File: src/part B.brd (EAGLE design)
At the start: 41 x 75.5 mm, 0 parts

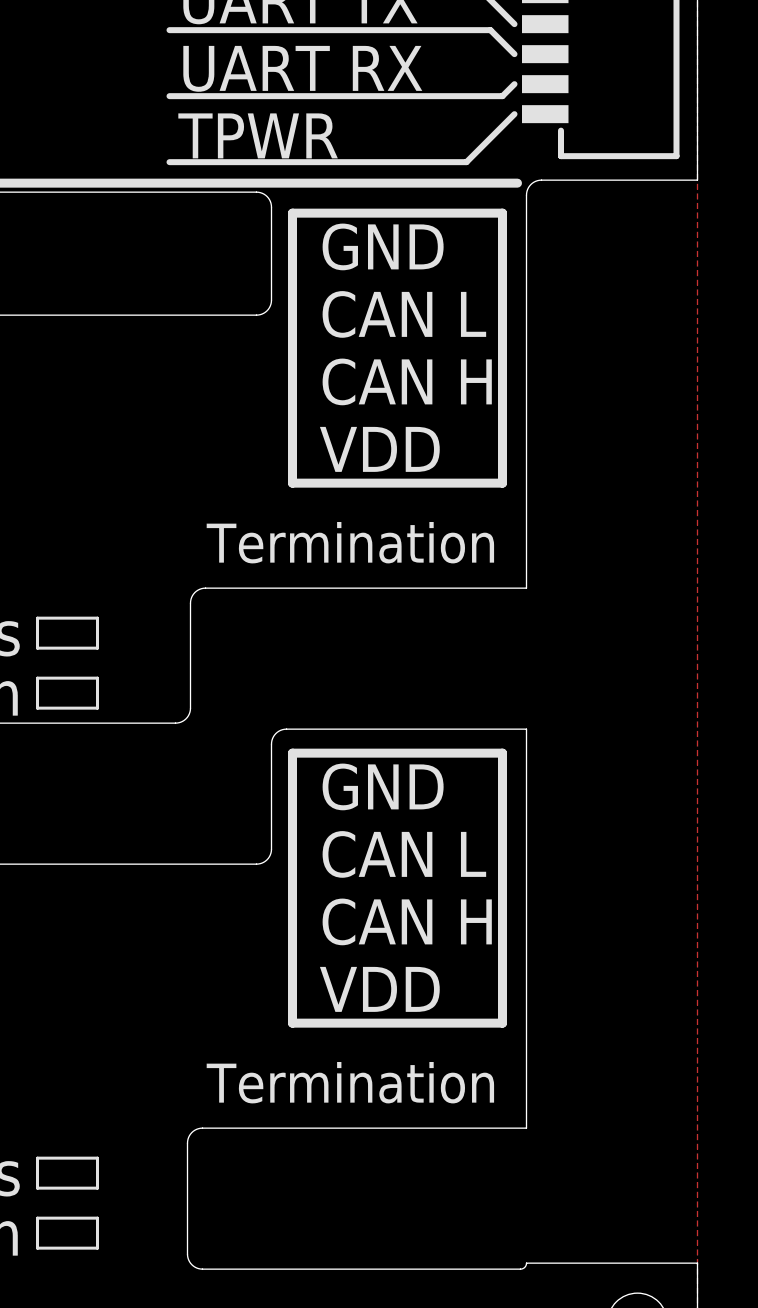
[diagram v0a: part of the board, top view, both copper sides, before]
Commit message: Minor tweaks
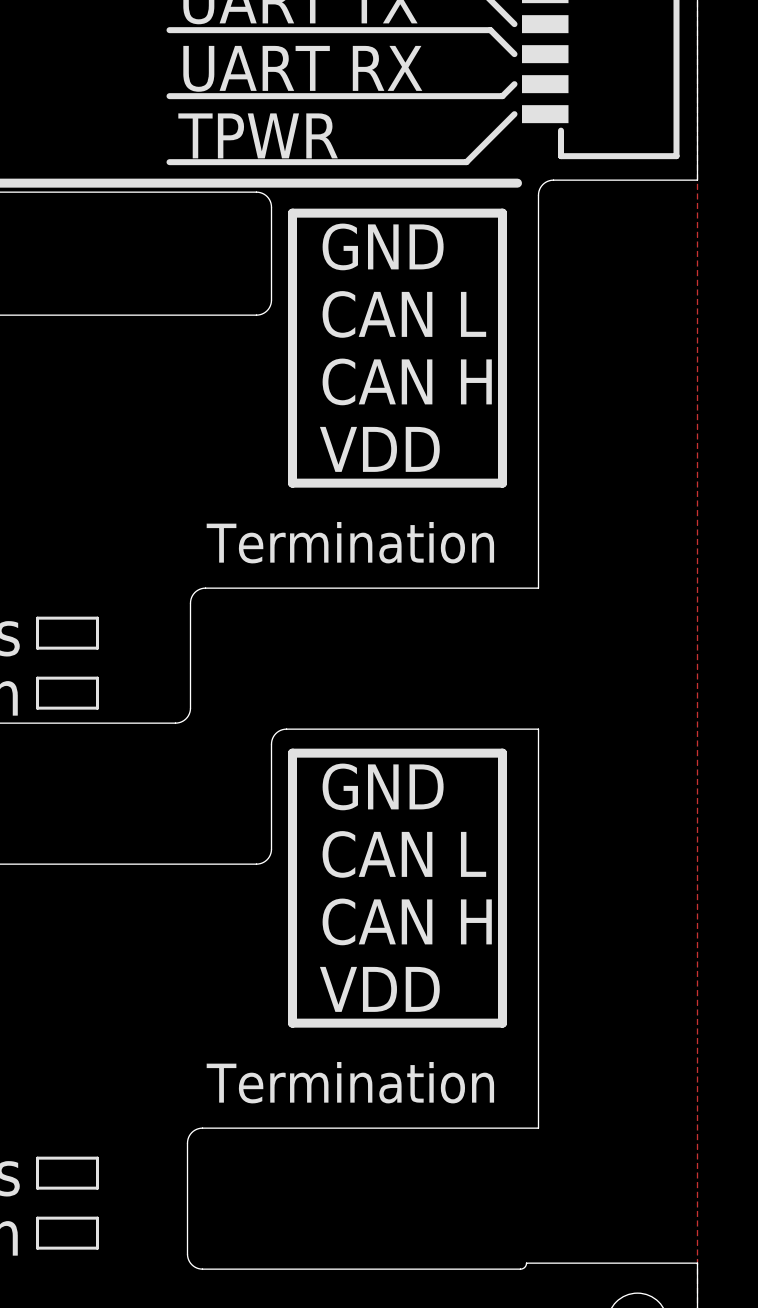
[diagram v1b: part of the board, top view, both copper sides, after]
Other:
- outline, holes or cut-outs redrawn
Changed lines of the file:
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@@
 <setting verticaltext="up"/>
 </settings>
-<grid distance="1" unitdist="mm" unit="mm" style="lines" multiple="1" display="yes" altdistance="5" altunitdist="mil" altunit="mil"/>
+<grid distance="0.4" unitdist="mm" unit="mm" style="lines" multiple="1" display="yes" altdistance="5" altunitdist="mil" altunit="mil"/>
 <layers>
-<layer number="1" name="Top" color="4" fill="1" visible="yes" active="yes"/>
+<layer number="1" name="Top" color="4" fill="1" visible="no" active="yes"/>
 <layer number="2" name="Route2" color="16" fill="1" visible="no" active="no"/>
 <layer number="3" name="Route3" color="17" fill="1" visible="no" active="no"/>
@@
 <layer number="14" name="Route14" color="22" fill="1" visible="no" active="no"/>
 <layer number="15" name="Route15" color="23" fill="1" visible="no" active="no"/>
-<layer number="16" name="Bottom" color="1" fill="1" visible="yes" active="yes"/>
-<layer number="17" name="Pads" color="2" fill="1" visible="yes" active="yes"/>
-<layer number="18" name="Vias" color="2" fill="1" visible="yes" active="yes"/>
+<layer number="16" name="Bottom" color="1" fill="1" visible="no" active="yes"/>
+<layer number="17" name="Pads" color="2" fill="1" visible="no" active="yes"/>
+<layer number="18" name="Vias" color="2" fill="1" visible="no" active="yes"/>
 <layer number="19" name="Unrouted" color="6" fill="1" visible="no" active="yes"/>
-<layer number="20" name="Dimension" color="24" fill="1" visible="no" active="yes"/>
-<layer number="21" name="tPlace" color="7" fill="1" visible="yes" active="yes"/>
-<layer number="22" name="bPlace" color="7" fill="1" visible="yes" active="yes"/>
-<layer number="23" name="tOrigins" color="15" fill="1" visible="yes" active="yes"/>
-<layer number="24" name="bOrigins" color="15" fill="1" visible="yes" active="yes"/>
-<layer number="25" name="tNames" color="7" fill="1" visible="yes" active="yes"/>
-<layer number="26" name="bNames" color="7" fill="1" visible="yes" active="yes"/>
-<layer number="27" name="tValues" color="7" fill="1" visible="yes" active="yes"/>
-<layer number="28" name="bValues" color="7" fill="1" visible="yes" active="yes"/>
-<layer number="29" name="tStop" color="7" fill="3" visible="yes" active="yes"/>
-<layer number="30" name="bStop" color="7" fill="6" visible="yes" active="yes"/>
+<layer number="20" name="Dimension" color="24" fill="1" visible="yes" active="yes"/>
+<layer number="21" name="tPlace" color="7" fill="1" visible="no" active="yes"/>
+<layer number="22" name="bPlace" color="7" fill="1" visible="no" active="yes"/>
+<layer number="23" name="tOrigins" color="15" fill="1" visible="no" active="yes"/>
+<layer number="24" name="bOrigins" color="15" fill="1" visible="no" active="yes"/>
+<layer number="25" name="tNames" color="7" fill="1" visible="no" active="yes"/>
+<layer number="26" name="bNames" color="7" fill="1" visible="no" active="yes"/>
+<layer number="27" name="tValues" color="7" fill="1" visible="no" active="yes"/>
+<layer number="28" name="bValues" color="7" fill="1" visible="no" active="yes"/>
+<layer number="29" name="tStop" color="7" fill="3" visible="no" active="yes"/>
+<layer number="30" name="bStop" color="7" fill="6" visible="no" active="yes"/>
 <layer number="31" name="tCream" color="7" fill="4" visible="no" active="yes"/>
 <layer number="32" name="bCream" color="7" fill="5" visible="no" active="yes"/>
@@
 <layer number="37" name="tTest" color="7" fill="1" visible="no" active="yes"/>
 <layer number="38" name="bTest" color="7" fill="1" visible="no" active="yes"/>
-<layer number="39" name="tKeepout" color="4" fill="11" visible="yes" active="yes"/>
-<layer number="40" name="bKeepout" color="1" fill="11" visible="yes" active="yes"/>
-<layer number="41" name="tRestrict" color="4" fill="10" visible="yes" active="yes"/>
-<layer number="42" name="bRestrict" color="1" fill="10" visible="yes" active="yes"/>
-<layer number="43" name="vRestrict" color="2" fill="10" visible="yes" active="yes"/>
+<layer number="39" name="tKeepout" color="4" fill="11" visible="no" active="yes"/>
+<layer number="40" name="bKeepout" color="1" fill="11" visible="no" active="yes"/>
+<layer number="41" name="tRestrict" color="4" fill="10" visible="no" active="yes"/>
+<layer number="42" name="bRestrict" color="1" fill="10" visible="no" active="yes"/>
+<layer number="43" name="vRestrict" color="2" fill="10" visible="no" active="yes"/>
 <layer number="44" name="Drills" color="7" fill="1" visible="no" active="yes"/>
-<layer number="45" name="Holes" color="7" fill="1" visible="yes" active="yes"/>
+<layer number="45" name="Holes" color="7" fill="1" visible="no" active="yes"/>
 <layer number="46" name="Milling" color="3" fill="1" visible="no" active="yes"/>
 <layer number="47" name="Measures" color="7" fill="1" visible="no" active="yes"/>
-<layer number="48" name="Document" color="7" fill="1" visible="yes" active="yes"/>
-<layer number="49" name="Reference" color="7" fill="1" visible="yes" active="yes"/>
+<layer number="48" name="Document" color="7" fill="1" visible="no" active="yes"/>
+<layer number="49" name="Reference" color="7" fill="1" visible="no" active="yes"/>
 <layer number="50" name="dxf" color="7" fill="1" visible="no" active="no"/>
-<layer number="51" name="tDocu" color="7" fill="1" visible="yes" active="yes"/>
-<layer number="52" name="bDocu" color="7" fill="1" visible="yes" active="yes"/>
+<layer number="51" name="tDocu" color="7" fill="1" visible="no" active="yes"/>
+<layer number="52" name="bDocu" color="7" fill="1" visible="no" active="yes"/>
 <layer number="53" name="tGND_GNDA" color="7" fill="9" visible="no" active="no"/>
 <layer number="54" name="bGND_GNDA" color="1" fill="9" visible="no" active="no"/>
@@
 <layer number="106" name="bPlate" color="7" fill="1" visible="no" active="yes"/>
 <layer number="107" name="Crop" color="7" fill="1" visible="no" active="yes"/>
-<layer number="108" name="fp8" color="7" fill="1" visible="yes" active="yes"/>
+<layer number="108" name="fp8" color="7" fill="1" visible="no" active="yes"/>
 <layer number="109" name="fp9" color="7" fill="1" visible="no" active="yes"/>
 <layer number="110" name="fp0" color="7" fill="1" visible="no" active="yes"/>
@@
 <hole x="35" y="-2" drill="2"/>
 <hole x="-2" y="-2" drill="2"/>
-<wire x1="31.3" y1="17.8" x2="23.3" y2="17.8" width="0.01" layer="20"/>
+<wire x1="31.7" y1="17.8" x2="23.3" y2="17.8" width="0.01" layer="20"/>
 <wire x1="23.3" y1="17.8" x2="22.8" y2="17.3" width="0.01" layer="20" curve="90"/>
 <wire x1="22.8" y1="17.3" x2="22.8" y2="13.8" width="0.01" layer="20"/>
@@
 <wire x1="20.1" y1="18.5" x2="19.6" y2="18" width="0.01" layer="20" curve="-90"/>
 <wire x1="19.6" y1="18" x2="12.5" y2="18" width="0.01" layer="20"/>
-<wire x1="31.3" y1="22.5" x2="20.6" y2="22.5" width="0.01" layer="20"/>
+<wire x1="31.7" y1="22.5" x2="20.6" y2="22.5" width="0.01" layer="20"/>
 <wire x1="20.6" y1="22.5" x2="20.1" y2="22" width="0.01" layer="20" curve="90"/>
 <wire x1="22.8" y1="32.1" x2="22.8" y2="35.2" width="0.01" layer="20"/>
@@
 <wire x1="12.5" y1="31.6" x2="22.3" y2="31.6" width="0.01" layer="20"/>
 <wire x1="22.3" y1="31.6" x2="22.8" y2="32.1" width="0.01" layer="20" curve="90"/>
-<wire x1="31.3" y1="4.5" x2="20.5" y2="4.5" width="0.01" layer="20"/>
+<wire x1="31.7" y1="4.5" x2="20.5" y2="4.5" width="0.01" layer="20"/>
 <wire x1="20.5" y1="4.5" x2="20" y2="4" width="0.01" layer="20" curve="90"/>
 <wire x1="20" y1="4" x2="20" y2="0.3" width="0.01" layer="20"/>
@@
 <wire x1="22.9" y1="52.5" x2="23.4" y2="52" width="0.01" layer="20" curve="90"/>
 <wire x1="23.4" y1="52" x2="37" y2="52" width="0.01" layer="20"/>
-<wire x1="31.3" y1="35.6" x2="31.3" y2="22.5" width="0.01" layer="20"/>
-<wire x1="31.3" y1="17.8" x2="31.3" y2="4.5" width="0.01" layer="20"/>
-<wire x1="31.3" y1="35.6" x2="31.8" y2="36.1" width="0.01" layer="20" curve="-90"/>
-<wire x1="31.8" y1="36.1" x2="37" y2="36.1" width="0.01" layer="20"/>
+<wire x1="31.7" y1="22.5" x2="31.7" y2="35.6" width="0.01" layer="20"/>
+<wire x1="31.7" y1="35.6" x2="32.2" y2="36.1" width="0.01" layer="20" curve="-90"/>
+<wire x1="32.2" y1="36.1" x2="37" y2="36.1" width="0.01" layer="20"/>
+<wire x1="31.7" y1="17.8" x2="31.7" y2="4.5" width="0.01" layer="20"/>
 <hole x="35" y="48.2" drill="2"/>
 <wire x1="-4" y1="-2" x2="-4" y2="69.5" width="0.01" layer="20"/>
